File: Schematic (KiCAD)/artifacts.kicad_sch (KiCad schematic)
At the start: 144 parts, among them J14 NAND_2, J15 NOR_3, J3 BIGBUF, J56 INVERT, J57 INVERT, J58 INVERT, J61 INVERT, J62 INVERT, J63 NOR_3, J64 NOR_3, J67 INVERT, J69 INVERT, K23 INVERT, K24 NAND_2, K61 NAND_3, K62 INVERT

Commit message: I fixed 2 errors in the letterless MMC5 tracing:
1. BK5 is a NAND-4 gate.  It was thought to be NAND-3 before.
2.  BL83 and BL96 signals got swapped here before.  They actually cross each other:

BL83 = "PPU_RW_Mode_%0x_Access"
BL96 = "+ExRAM_Mode_$0x"

This propagated out to several changes in the schematic.
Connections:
- net at H45. (X): now also H66. (X); no longer H44. (X)
- net at H66. (X): now also H63. (X); no longer H45. (X)
- net at L61. (X): now also J15. (X); no longer L60. (X)
- net at J15. (X): now also L19. (X); no longer L61. (X)
- net at G47. (X): now also G46. (X); no longer G51. (X)
- net at H71. (X): now also H74. (X); no longer H70. (X)
- net at G63. (X): now also G64. (X); no longer G62. (X)
- net at G64. (X): now also G65. (X); no longer G63. (X)
- net at H74. (X): now also H75. (X); no longer H71. (X)
- net at H73. (X): now also H72. (X); no longer H74. (X)
- net at H47. (X): now also H46. (X); no longer H74. (X)
- net at H75. (X): now also H80. (/Q3); no longer H74. (X)
- net at G58. (X): now also G57. (X); no longer G34. (X)
- net at G59. (X): now also G69. (/Q3); no longer G58. (X)
- net at G55. (X): now also G54. (X); no longer G58. (X)
- net at G57. (X): now also G56. (X); no longer G58. (X)
- net at H58. (X): now also H80. (/Q3); no longer H57. (X)
- net at J62. (X): now also J63. (X); no longer J61. (X)
- net at G96. (X): now also F25. (X); no longer G86. (X)
- net at H43. (X): now also H42. (X); no longer H57. (X)
- net at B36. (X): now also B35. (X); no longer B37. (X)
- net at C4. (X): now also C3. (X); no longer C5. (X)
- net at G40. (X): now also G41. (X); no longer G39. (X)
- net at H49. (X): now also H50. (X); no longer H48. (X)
- net at B32. (X): now also B31. (X); no longer B33. (X)
- net at B27. (X): now also B28. (X); no longer B26. (X)
- net at H50. (X): now also H51. (X); no longer H41. (X)
- net at H51. (X): now also H80. (/Q3); no longer H50. (X)
- net at L20. (X): now also J58. (X); no longer K23. (X)
- net at J58. (X): now also J57. (X); no longer L20. (X)
- net at B93. (X): now also B69. (X); no longer A76. (X)
- net at G38. (X): now also G41. (X); no longer G37. (X)
- net at G50. (X): now also G51. (X); no longer G49. (X)
- net at H59. (X): now also J69. (X); no longer H81. (X)
- net at J56. (X): now also K62. (X); no longer J57. (X)
- net at K62. (X): now also K61. (X); no longer J56. (X)
- net at A20. (X): now also A21. (X); no longer A19. (X)
- net at B96. (X): now also B95. (X); no longer B97. (X)
- net at G51. (X): now also G32. (X); no longer G50. (X)
- net at G52. (X): now also G69. (/Q3); no longer G51. (X)
- net at G32. (X): now also G31. (X); no longer G51. (X)
- net at H57. (X): now also H56. (X); no longer H54. (X)
- net at H56. (X): now also H55. (X); no longer H57. (X)
- net at E32. (X): now also E31. (X); no longer E33. (X)
- net at L19. (X): now also J3. (X); no longer J15. (X)
- net at G36. (X): now also G64. (X); no longer G35. (X)
- net at H67. (X): now also H66. (X); no longer H80. (/Q3)
- net at J63. (X): now also J64. (X); no longer J62. (X)
- net at C29. (X): now also B69. (X); no longer C30. (X)
- net at G61. (X): now also G64. (X); no longer G60. (X)
- net at B28. (X): now also B29. (X); no longer B27. (X)
- net at E66. (X): now also D43. (X); no longer E54. (X)
- net at K24. (X): now also K23. (X); no longer J14. (X)
- net at G65. (X): now also G69. (/Q3); no longer G64. (X)
- net at H65. (X): now also H64. (X); no longer H66. (X)
- net at G42. (X): now also G41. (X); no longer G69. (/Q3)
- net at B35. (X): now also B34. (X); no longer B36. (X)
- new net: H44. (X), H45. (X)
- new net: L60. (X), L61. (X)
- new net: G47. (X), G51. (X)
- new net: H38. (X), H48. (X), H53. (X), H55. (X), H61. (X), H62. (X), H64. (X), H69. (X), H70. (X), H72. (X)
- new net: H70. (X), H71. (X)
- new net: H69. (X), H70. (X)
- new net: H38. (X), H39. (X), H40. (X), H42. (X), H44. (X), H46. (X)
- new net: G62. (X), G63. (X)
- new net: H73. (X), H74. (X)
- new net: H47. (X), H74. (X)
- new net: G34. (X), G58. (X)
- new net: G58. (X), G59. (X)
- new net: G55. (X), G58. (X)
- new net: H57. (X), H58. (X)
- new net: J61. (X), J62. (X)
- new net: G86. (X), G96. (X)
- new net: F25. (X), G96. (X)
- new net: H43. (X), H57. (X)
- new net: B36. (X), B37. (X)
- new net: C4. (X), C5. (X)
- new net: G30. (X), G39. (X), G46. (X), G48. (X), G49. (X), G53. (X), G54. (X), G56. (X), G60. (X), G62. (X)
- new net: G39. (X), G40. (X)
- new net: H61. (X), H62. (X)
- new net: H62. (X), H63. (X)
- new net: H48. (X), H49. (X)
- new net: B32. (X), B33. (X)
- new net: B26. (X), B27. (X)
- new net: H41. (X), H50. (X)
- new net: K23. (X), L20. (X)
- new net: A76. (X), B93. (X)
- new net: G37. (X), G38. (X)
- new net: G49. (X), G50. (X)
- new net: G48. (X), G49. (X)
- new net: H59. (X), H81. (X)
- new net: J56. (X), J57. (X)
- new net: A19. (X), A20. (X)
- new net: A20. (X), A21. (X)
- new net: B96. (X), B97. (X)
- new net: G51. (X), G52. (X)
- new net: G53. (X), G56. (X)
- new net: H54. (X), H57. (X)
- new net: E32. (X), E33. (X)
- new net: G29. (X), G30. (X), G31. (X), G33. (X), G35. (X), G37. (X)
- new net: G35. (X), G36. (X)
- new net: E31. (X), F6.1. (X)
- new net: H67. (X), H80. (/Q3)
- new net: J63. (X), J64. (X)
- new net: C29. (X), C30. (X)
- new net: G43. (X), G44. (X)
- new net: C2. (X), C3. (X)
- new net: G60. (X), G61. (X)
- new net: E54. (X), E66. (X)
- new net: D43. (X), E66. (X)
- new net: J14. (X), K24. (X)
- new net: B28. (X), B29. (X)
- new net: H77. (X), H78. (X)
- new net: D44. (X), J69. (X)
- new net: H65. (X), H66. (X)
- new net: G42. (X), G69. (/Q3)

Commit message: Schematic and SVG Updates
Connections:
- net at H45. (X): now also H66. (X); no longer H44. (X)
- net at H66. (X): now also H63. (X); no longer H45. (X)
- net at L61. (X): now also J15. (X); no longer L60. (X)
- net at J15. (X): now also L19. (X); no longer L61. (X)
- net at G47. (X): now also G46. (X); no longer G51. (X)
- net at H71. (X): now also H74. (X); no longer H70. (X)
- net at G63. (X): now also G64. (X); no longer G62. (X)
- net at G64. (X): now also G65. (X); no longer G63. (X)
- net at H74. (X): now also H75. (X); no longer H71. (X)
- net at H73. (X): now also H72. (X); no longer H74. (X)
- net at H47. (X): now also H46. (X); no longer H74. (X)
- net at H75. (X): now also H80. (/Q3); no longer H74. (X)
- net at G58. (X): now also G57. (X); no longer G34. (X)
- net at G59. (X): now also G69. (/Q3); no longer G58. (X)
- net at G55. (X): now also G54. (X); no longer G58. (X)
- net at G57. (X): now also G56. (X); no longer G58. (X)
- net at H58. (X): now also H80. (/Q3); no longer H57. (X)
- net at J62. (X): now also J63. (X); no longer J61. (X)
- net at G96. (X): now also F25. (X); no longer G86. (X)
- net at H43. (X): now also H42. (X); no longer H57. (X)
- net at B36. (X): now also B35. (X); no longer B37. (X)
- net at C4. (X): now also C3. (X); no longer C5. (X)
- net at G40. (X): now also G41. (X); no longer G39. (X)
- net at H49. (X): now also H50. (X); no longer H48. (X)
- net at B32. (X): now also B31. (X); no longer B33. (X)
- net at B27. (X): now also B28. (X); no longer B26. (X)
- net at H50. (X): now also H51. (X); no longer H41. (X)
- net at H51. (X): now also H80. (/Q3); no longer H50. (X)
- net at L20. (X): now also J58. (X); no longer K23. (X)
- net at J58. (X): now also J57. (X); no longer L20. (X)
- net at B93. (X): now also B69. (X); no longer A76. (X)
- net at G38. (X): now also G41. (X); no longer G37. (X)
- net at G50. (X): now also G51. (X); no longer G49. (X)
- net at H59. (X): now also J69. (X); no longer H81. (X)
- net at J56. (X): now also K62. (X); no longer J57. (X)
- net at K62. (X): now also K61. (X); no longer J56. (X)
- net at A20. (X): now also A21. (X); no longer A19. (X)
- net at B96. (X): now also B95. (X); no longer B97. (X)
- net at G51. (X): now also G32. (X); no longer G50. (X)
- net at G52. (X): now also G69. (/Q3); no longer G51. (X)
- net at G32. (X): now also G31. (X); no longer G51. (X)
- net at H57. (X): now also H56. (X); no longer H54. (X)
- net at H56. (X): now also H55. (X); no longer H57. (X)
- net at E32. (X): now also E31. (X); no longer E33. (X)
- net at L19. (X): now also J3. (X); no longer J15. (X)
- net at G36. (X): now also G64. (X); no longer G35. (X)
- net at H67. (X): now also H66. (X); no longer H80. (/Q3)
- net at J63. (X): now also J64. (X); no longer J62. (X)
- net at C29. (X): now also B69. (X); no longer C30. (X)
- net at G61. (X): now also G64. (X); no longer G60. (X)
- net at B28. (X): now also B29. (X); no longer B27. (X)
- net at E66. (X): now also D43. (X); no longer E54. (X)
- net at K24. (X): now also K23. (X); no longer J14. (X)
- net at G65. (X): now also G69. (/Q3); no longer G64. (X)
- net at H65. (X): now also H64. (X); no longer H66. (X)
- net at G42. (X): now also G41. (X); no longer G69. (/Q3)
- net at B35. (X): now also B34. (X); no longer B36. (X)
- new net: H44. (X), H45. (X)
- new net: L60. (X), L61. (X)
- new net: G47. (X), G51. (X)
- new net: H38. (X), H48. (X), H53. (X), H55. (X), H61. (X), H62. (X), H64. (X), H69. (X), H70. (X), H72. (X)
- new net: H70. (X), H71. (X)
- new net: H69. (X), H70. (X)
- new net: H38. (X), H39. (X), H40. (X), H42. (X), H44. (X), H46. (X)
- new net: G62. (X), G63. (X)
- new net: H73. (X), H74. (X)
- new net: H47. (X), H74. (X)
- new net: G34. (X), G58. (X)
- new net: G58. (X), G59. (X)
- new net: G55. (X), G58. (X)
- new net: H57. (X), H58. (X)
- new net: J61. (X), J62. (X)
- new net: G86. (X), G96. (X)
- new net: F25. (X), G96. (X)
- new net: H43. (X), H57. (X)
- new net: B36. (X), B37. (X)
- new net: C4. (X), C5. (X)
- new net: G30. (X), G39. (X), G46. (X), G48. (X), G49. (X), G53. (X), G54. (X), G56. (X), G60. (X), G62. (X)
- new net: G39. (X), G40. (X)
- new net: H61. (X), H62. (X)
- new net: H62. (X), H63. (X)
- new net: H48. (X), H49. (X)
- new net: B32. (X), B33. (X)
- new net: B26. (X), B27. (X)
- new net: H41. (X), H50. (X)
- new net: K23. (X), L20. (X)
- new net: A76. (X), B93. (X)
- new net: G37. (X), G38. (X)
- new net: G49. (X), G50. (X)
- new net: G48. (X), G49. (X)
- new net: H59. (X), H81. (X)
- new net: J56. (X), J57. (X)
- new net: A19. (X), A20. (X)
- new net: A20. (X), A21. (X)
- new net: B96. (X), B97. (X)
- new net: G51. (X), G52. (X)
- new net: G53. (X), G56. (X)
- new net: H54. (X), H57. (X)
- new net: E32. (X), E33. (X)
- new net: G29. (X), G30. (X), G31. (X), G33. (X), G35. (X), G37. (X)
- new net: G35. (X), G36. (X)
- new net: E31. (X), F6.1. (X)
- new net: H67. (X), H80. (/Q3)
- new net: J63. (X), J64. (X)
- new net: C29. (X), C30. (X)
- new net: G43. (X), G44. (X)
- new net: C2. (X), C3. (X)
- new net: G60. (X), G61. (X)
- new net: E54. (X), E66. (X)
- new net: D43. (X), E66. (X)
- new net: J14. (X), K24. (X)
- new net: B28. (X), B29. (X)
- new net: H77. (X), H78. (X)
- new net: D44. (X), J69. (X)
- new net: H65. (X), H66. (X)
- new net: G42. (X), G69. (/Q3)

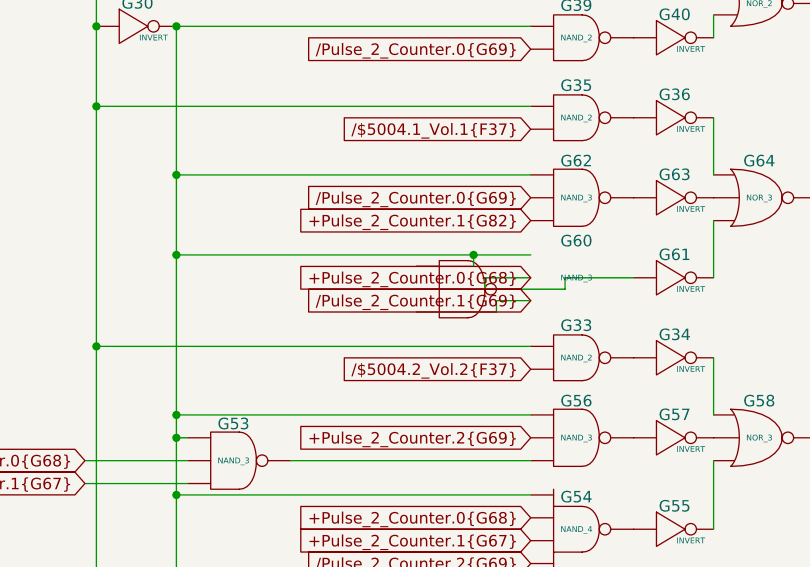
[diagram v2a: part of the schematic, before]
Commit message: Schematic and SVG Updates
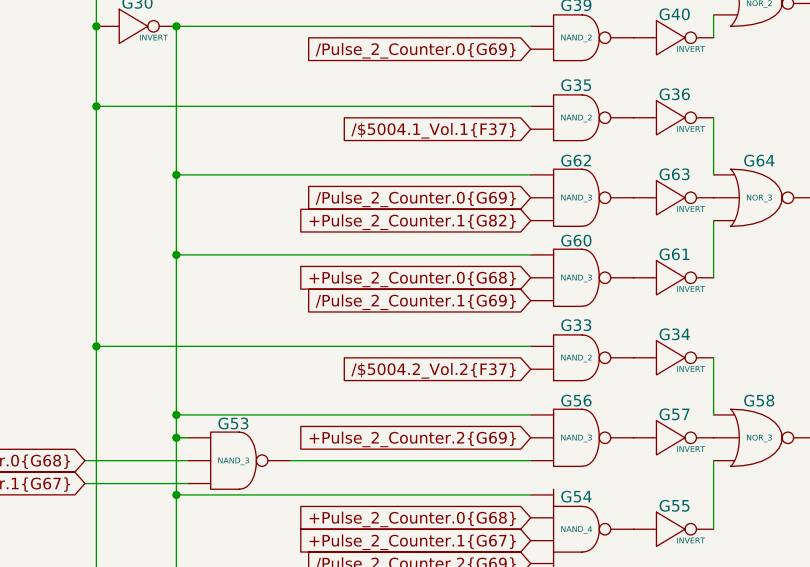
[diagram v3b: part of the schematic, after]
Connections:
- net at H45. (X): now also H66. (X); no longer H44. (X)
- net at H66. (X): now also H63. (X); no longer H45. (X)
- net at L61. (X): now also J15. (X); no longer L60. (X)
- net at J15. (X): now also L19. (X); no longer L61. (X)
- net at G47. (X): now also G46. (X); no longer G51. (X)
- net at H71. (X): now also H74. (X); no longer H70. (X)
- net at G63. (X): now also G64. (X); no longer G62. (X)
- net at G64. (X): now also G65. (X); no longer G63. (X)
- net at H74. (X): now also H75. (X); no longer H71. (X)
- net at H73. (X): now also H72. (X); no longer H74. (X)
- net at H47. (X): now also H46. (X); no longer H74. (X)
- net at H75. (X): now also H80. (/Q3); no longer H74. (X)
- net at G58. (X): now also G57. (X); no longer G34. (X)
- net at G59. (X): now also G69. (/Q3); no longer G58. (X)
- net at G55. (X): now also G54. (X); no longer G58. (X)
- net at G57. (X): now also G56. (X); no longer G58. (X)
- net at H58. (X): now also H80. (/Q3); no longer H57. (X)
- net at J62. (X): now also J63. (X); no longer J61. (X)
- net at G96. (X): now also F25. (X); no longer G86. (X)
- net at H43. (X): now also H42. (X); no longer H57. (X)
- net at B36. (X): now also B35. (X); no longer B37. (X)
- net at C4. (X): now also C3. (X); no longer C5. (X)
- net at G40. (X): now also G41. (X); no longer G39. (X)
- net at H49. (X): now also H50. (X); no longer H48. (X)
- net at B32. (X): now also B31. (X); no longer B33. (X)
- net at B27. (X): now also B28. (X); no longer B26. (X)
- net at H50. (X): now also H51. (X); no longer H41. (X)
- net at H51. (X): now also H80. (/Q3); no longer H50. (X)
- net at L20. (X): now also J58. (X); no longer K23. (X)
- net at J58. (X): now also J57. (X); no longer L20. (X)
- net at B93. (X): now also B69. (X); no longer A76. (X)
- net at G38. (X): now also G41. (X); no longer G37. (X)
- net at G50. (X): now also G51. (X); no longer G49. (X)
- net at H59. (X): now also J69. (X); no longer H81. (X)
- net at J56. (X): now also K62. (X); no longer J57. (X)
- net at K62. (X): now also K61. (X); no longer J56. (X)
- net at A20. (X): now also A21. (X); no longer A19. (X)
- net at B96. (X): now also B95. (X); no longer B97. (X)
- net at G51. (X): now also G32. (X); no longer G50. (X)
- net at G52. (X): now also G69. (/Q3); no longer G51. (X)
- net at G32. (X): now also G31. (X); no longer G51. (X)
- net at H57. (X): now also H56. (X); no longer H54. (X)
- net at H56. (X): now also H55. (X); no longer H57. (X)
- net at E32. (X): now also E31. (X); no longer E33. (X)
- net at L19. (X): now also J3. (X); no longer J15. (X)
- net at G36. (X): now also G64. (X); no longer G35. (X)
- net at H67. (X): now also H66. (X); no longer H80. (/Q3)
- net at J63. (X): now also J64. (X); no longer J62. (X)
- net at C29. (X): now also B69. (X); no longer C30. (X)
- net at G61. (X): now also G64. (X); no longer G60. (X)
- net at B28. (X): now also B29. (X); no longer B27. (X)
- net at E66. (X): now also D43. (X); no longer E54. (X)
- net at K24. (X): now also K23. (X); no longer J14. (X)
- net at G65. (X): now also G69. (/Q3); no longer G64. (X)
- net at H65. (X): now also H64. (X); no longer H66. (X)
- net at G42. (X): now also G41. (X); no longer G69. (/Q3)
- net at B35. (X): now also B34. (X); no longer B36. (X)
- new net: H44. (X), H45. (X)
- new net: L60. (X), L61. (X)
- new net: G47. (X), G51. (X)
- new net: H38. (X), H48. (X), H53. (X), H55. (X), H61. (X), H62. (X), H64. (X), H69. (X), H70. (X), H72. (X)
- new net: H70. (X), H71. (X)
- new net: H69. (X), H70. (X)
- new net: H38. (X), H39. (X), H40. (X), H42. (X), H44. (X), H46. (X)
- new net: G62. (X), G63. (X)
- new net: H73. (X), H74. (X)
- new net: H47. (X), H74. (X)
- new net: G34. (X), G58. (X)
- new net: G58. (X), G59. (X)
- new net: G55. (X), G58. (X)
- new net: H57. (X), H58. (X)
- new net: J61. (X), J62. (X)
- new net: G86. (X), G96. (X)
- new net: F25. (X), G96. (X)
- new net: H43. (X), H57. (X)
- new net: B36. (X), B37. (X)
- new net: C4. (X), C5. (X)
- new net: G30. (X), G39. (X), G46. (X), G48. (X), G49. (X), G53. (X), G54. (X), G56. (X), G60. (X), G62. (X)
- new net: G39. (X), G40. (X)
- new net: H61. (X), H62. (X)
- new net: H62. (X), H63. (X)
- new net: H48. (X), H49. (X)
- new net: B32. (X), B33. (X)
- new net: G60. (X), G61. (X)
- new net: B26. (X), B27. (X)
- new net: H41. (X), H50. (X)
- new net: K23. (X), L20. (X)
- new net: A76. (X), B93. (X)
- new net: G37. (X), G38. (X)
- new net: G49. (X), G50. (X)
- new net: G48. (X), G49. (X)
- new net: H59. (X), H81. (X)
- new net: J56. (X), J57. (X)
- new net: A19. (X), A20. (X)
- new net: A20. (X), A21. (X)
- new net: B96. (X), B97. (X)
- new net: G51. (X), G52. (X)
- new net: G53. (X), G56. (X)
- new net: H54. (X), H57. (X)
- new net: E32. (X), E33. (X)
- new net: G29. (X), G30. (X), G31. (X), G33. (X), G35. (X), G37. (X)
- new net: G35. (X), G36. (X)
- new net: E31. (X), F6.1. (X)
- new net: H67. (X), H80. (/Q3)
- new net: J63. (X), J64. (X)
- new net: C29. (X), C30. (X)
- new net: G43. (X), G44. (X)
- new net: C2. (X), C3. (X)
- new net: E54. (X), E66. (X)
- new net: D43. (X), E66. (X)
- new net: J14. (X), K24. (X)
- new net: B28. (X), B29. (X)
- new net: H77. (X), H78. (X)
- new net: D44. (X), J69. (X)
- new net: H65. (X), H66. (X)
- new net: G42. (X), G69. (/Q3)
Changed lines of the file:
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@@
 	)
 	(junction
-		(at 260.35 176.53)
-		(diameter 0)
-		(color 0 0 0 0)
-	)
-	(junction
 		(at 74.93 102.87)
 		(diameter 0)
@@
 	(wire
 		(pts
-			(xy 260.35 177.8) (xy 254 177.8)
-		)
-		(stroke
-			(width 0)
-			(type default)
-		)
-	)
-	(wire
-		(pts
 			(xy 332.74 62.23) (xy 321.31 62.23)
 		)
@@
 	(wire
 		(pts
-			(xy 262.89 181.61) (xy 262.89 182.88)
-		)
-		(stroke
-			(width 0)
-			(type default)
-		)
-	)
-	(wire
-		(pts
-			(xy 278.13 179.07) (xy 270.51 179.07)
-		)
-		(stroke
-			(width 0)
-			(type default)
-		)
-	)
-	(wire
-		(pts
 			(xy 97.79 49.53) (xy 97.79 44.45)
 		)
@@
 	(wire
 		(pts
-			(xy 227.33 176.53) (xy 260.35 176.53)
+			(xy 227.33 176.53) (xy 266.7 176.53)
 		)
 		(stroke
@@
 	(wire
 		(pts
-			(xy 262.89 182.88) (xy 254 182.88)
-		)
-		(stroke
-			(width 0)
-			(type default)
-		)
-	)
-	(wire
-		(pts
 			(xy 321.31 68.58) (xy 318.77 68.58)
 		)
@@
 	(wire
 		(pts
-			(xy 270.51 179.07) (xy 270.51 180.34)
-		)
-		(stroke
-			(width 0)
-			(type default)
-		)
-	)
-	(wire
-		(pts
 			(xy 287.02 68.58) (xy 287.02 74.93)
 		)
@@
 	(wire
 		(pts
-			(xy 270.51 180.34) (xy 265.43 180.34)
-		)
-		(stroke
-			(width 0)
-			(type default)
-		)
-	)
-	(wire
-		(pts
 			(xy 218.44 67.31) (xy 218.44 97.79)
 		)
@@
 	(wire
 		(pts
-			(xy 266.7 179.07) (xy 261.62 179.07)
-		)
-		(stroke
-			(width 0)
-			(type default)
-		)
-	)
-	(wire
-		(pts
 			(xy 74.93 147.32) (xy 74.93 149.86)
 		)
@@
 	(wire
 		(pts
-			(xy 261.62 180.34) (xy 254 180.34)
-		)
-		(stroke
-			(width 0)
-			(type default)
-		)
-	)
-	(wire
-		(pts
 			(xy 74.93 30.48) (xy 74.93 33.02)
 		)
@@
 	(wire
 		(pts
-			(xy 261.62 179.07) (xy 261.62 180.34)
-		)
-		(stroke
-			(width 0)
-			(type default)
-		)
-	)
-	(wire
-		(pts
 			(xy 218.44 143.51) (xy 266.7 143.51)
 		)
@@
 	(wire
 		(pts
-			(xy 266.7 181.61) (xy 262.89 181.61)
-		)
-		(stroke
-			(width 0)
-			(type default)
-		)
-	)
-	(wire
-		(pts
 			(xy 318.77 217.17) (xy 323.85 217.17)
 		)
@@
 	(wire
 		(pts
-			(xy 260.35 176.53) (xy 260.35 177.8)
-		)
-		(stroke
-			(width 0)
-			(type default)
-		)
-	)
-	(wire
-		(pts
 			(xy 86.36 138.43) (xy 86.36 139.7)
 		)
@@
 	(wire
 		(pts
-			(xy 266.7 176.53) (xy 260.35 176.53)
-		)
-		(stroke
-			(width 0)
-			(type default)
-		)
-	)
-	(wire
-		(pts
 			(xy 74.93 163.83) (xy 74.93 166.37)
 		)
@@
 	)
 	(symbol
+		(lib_name "NAND_3_11")
+		(lib_id "MMC5:NAND_3")
+		(at 271.78 179.07 0)
+		(unit 1)
+		(exclude_from_sim no)
+		(in_bom yes)
+		(on_board yes)
+		(dnp no)
+		(fields_autoplaced yes)
+		(property "Reference" "G60"
+			(at 271.78 174.244 0)
+			(do_not_autoplace yes)
+			(effects
+				(font
+					(size 1.27 1.27)
+				)
+				(justify top)
+			)
+		)
+		(property "Value" "NAND_3"
+			(at 271.78 179.07 0)
+			(do_not_autoplace yes)
+			(effects
+				(font
+					(size 0.635 0.635)
+				)
+			)
+		)
+		(property "Footprint" ""
+			(at 271.78 179.07 0)
+			(effects
+				(font
+					(size 1.27 1.27)
+				)
+				(hide yes)
+			)
+		)
+		(property "Datasheet" ""
+			(at 271.78 179.07 0)
+			(effects
+				(font
+					(size 1.27 1.27)
+				)
+				(hide yes)
+			)
+		)
+		(property "Description" ""
+			(at 271.78 179.07 0)
+			(effects
+				(font
+					(size 1.27 1.27)
+				)
+				(hide yes)
+			)
+		)
+		(pin ""
+		)
+		(pin ""
+		)
+		(pin ""
+		)
+		(pin ""
+		)
+		(instances
+			(project "MMC5"
+				(path "/46093bf6-f83e-4237-9ece-7350a682aff0/f2339e17-4f55-43f8-b207-f65123403db0"
+					(reference "G60")
+					(unit 1)
+				)
+			)
+		)
+	)
+	(symbol
 		(lib_name "INVERT_8")
 		(lib_id "MMC5:INVERT")
@@
 					(unit 1)
 				)
-			)
-		)
-	)
-	(symbol
-		(lib_name "NAND_3_18")
-		(lib_id "MMC5:NAND_3")
-		(at 259.08 180.34 0)
-		(unit 1)
-		(exclude_from_sim no)
-		(in_bom yes)
-		(on_board yes)
-		(dnp no)
-		(property "Reference" "G60"
-			(at 271.78 174.244 0)
-			(do_not_autoplace yes)
-			(effects
-				(font
-					(size 1.27 1.27)
-				)
-				(justify top)
-			)
-		)
-		(property "Value" "NAND_3"
-			(at 271.78 179.07 0)
-			(do_not_autoplace yes)
-			(effects
-				(font
-					(size 0.635 0.635)
-				)
-			)
-		)
-		(property "Footprint" ""
-			(at 259.08 180.34 0)
-			(effects
-				(font
-					(size 1.27 1.27)
-				)
-				(hide yes)
-			)
-		)
-		(property "Datasheet" ""
-			(at 259.08 180.34 0)
-			(effects
-				(font
-					(size 1.27 1.27)
-				)
-				(hide yes)
-			)
-		)
-		(property "Description" ""
-			(at 259.08 180.34 0)
-			(effects
-				(font
-					(size 1.27 1.27)
-				)
-				(hide yes)
-			)
-		)
-		(pin ""
-		)
-		(pin ""
-		)
-		(pin ""
-		)
-		(pin ""
-		)
-		(instances
-			(project "MMC5"
-				(path "/46093bf6-f83e-4237-9ece-7350a682aff0/f2339e17-4f55-43f8-b207-f65123403db0"
-					(reference "G60")
-					(unit 1)
-				)
